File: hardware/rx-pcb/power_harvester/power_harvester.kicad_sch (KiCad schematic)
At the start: 47 parts, among them J1 Conn_Coaxial_Small, J3 Conn_Coaxial_Small, J4 Conn_Coaxial_Small, J5 Conn_01x03_Pin

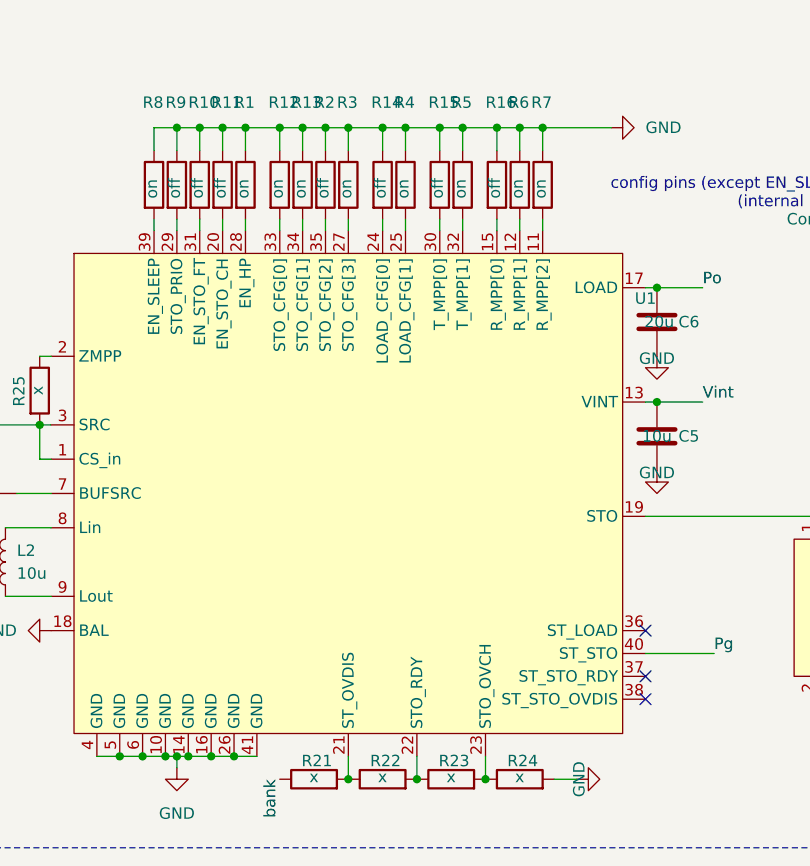
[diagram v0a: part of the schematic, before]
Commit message: minor harvester updates
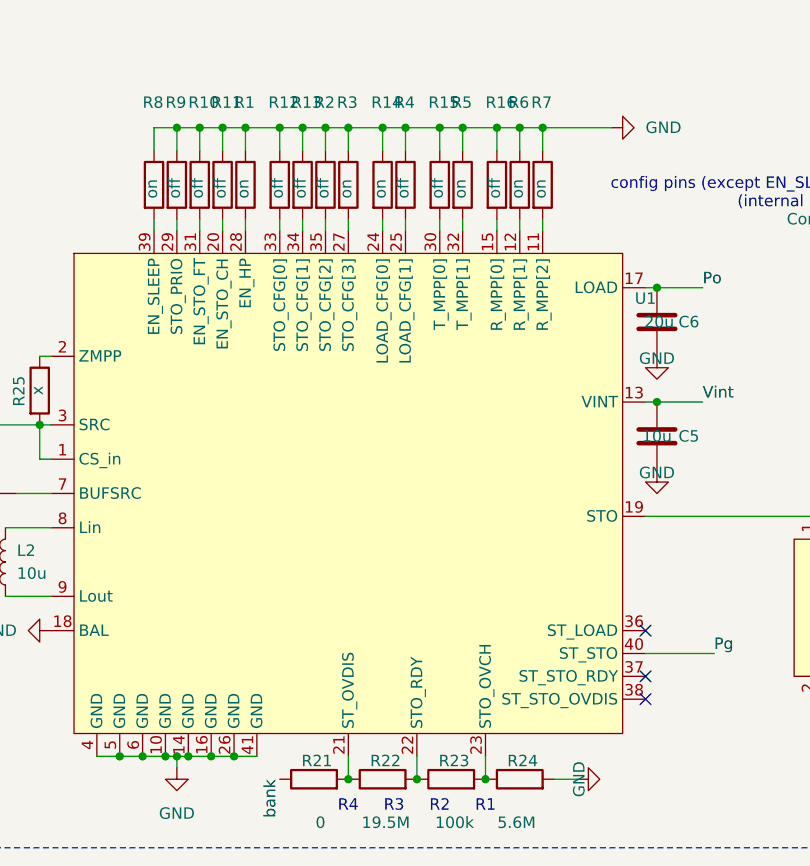
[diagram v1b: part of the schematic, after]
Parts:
- R12, R13, R4: value on -> off
- R14: value off -> on
- R21: value x -> 0
- R22: value x -> 19.5M
- R23: value x -> 100k
- R24: value x -> 5.6M
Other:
- note added: "R4 R3 R2 R1"
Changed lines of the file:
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@@
 		)
 	)
+	(text "R4     R3     R2     R1"
+		(exclude_from_sim no)
+		(at 78.74 188.468 0)
+		(effects
+			(font
+				(size 1.27 1.27)
+			)
+		)
+	)
 	(text "config pins (except EN_SLP) read floating as high\n(internal pull-up)"
 		(exclude_from_sim no)
@@
 			)
 		)
-		(property "Value" "x"
-			(at 75.438 185.166 90)
+		(property "Value" "19.5M"
+			(at 77.978 190.246 90)
 			(show_name no)
 			(do_not_autoplace no)
@@
 			)
 		)
-		(property "Value" "x"
-			(at 90.678 185.166 90)
+		(property "Value" "5.6M"
+			(at 91.948 190.246 90)
 			(show_name no)
 			(do_not_autoplace no)
@@
 			)
 		)
-		(property "Value" "x"
-			(at 83.058 185.166 90)
+		(property "Value" "100k"
+			(at 85.09 190.246 90)
 			(show_name no)
 			(do_not_autoplace no)
@@
 			)
 		)
-		(property "Value" "on"
+		(property "Value" "off"
 			(at 77.216 120.904 90)
 			(show_name no)
@@
 			)
 		)
-		(property "Value" "off"
+		(property "Value" "on"
 			(at 74.676 120.904 90)
 			(show_name no)
@@
 			)
 		)
-		(property "Value" "on"
+		(property "Value" "off"
 			(at 63.246 120.904 90)
 			(show_name no)
@@
 			)
 		)
-		(property "Value" "x"
-			(at 67.818 185.166 90)
+		(property "Value" "0"
+			(at 68.58 190.246 90)
 			(show_name no)
 			(do_not_autoplace no)
@@
 			)
 		)
-		(property "Value" "on"
+		(property "Value" "off"
 			(at 65.786 120.904 90)
 			(show_name no)
